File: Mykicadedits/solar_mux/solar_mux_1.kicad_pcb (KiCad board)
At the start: 2 copper layers, 122.9 x 145.3 mm, 26 parts, among them J1 Conn_01x14, U1 ASSR-1611, U10 ASSR-1611, U11 ASSR-1611, U12 ASSR-1611, U13 ASSR-1611, U14 ASSR-1611, U15 ASSR-1611, U16 ASSR-1611, U17 ASSR-1611, U2 ASSR-1611, U20 ASSR-1611, U21 ASSR-1611, U22 MCP23S17, U3 ASSR-1611, U4 ASSR-1611, U5 ASSR-1611, U6 ASSR-1611, U7 ASSR-1611

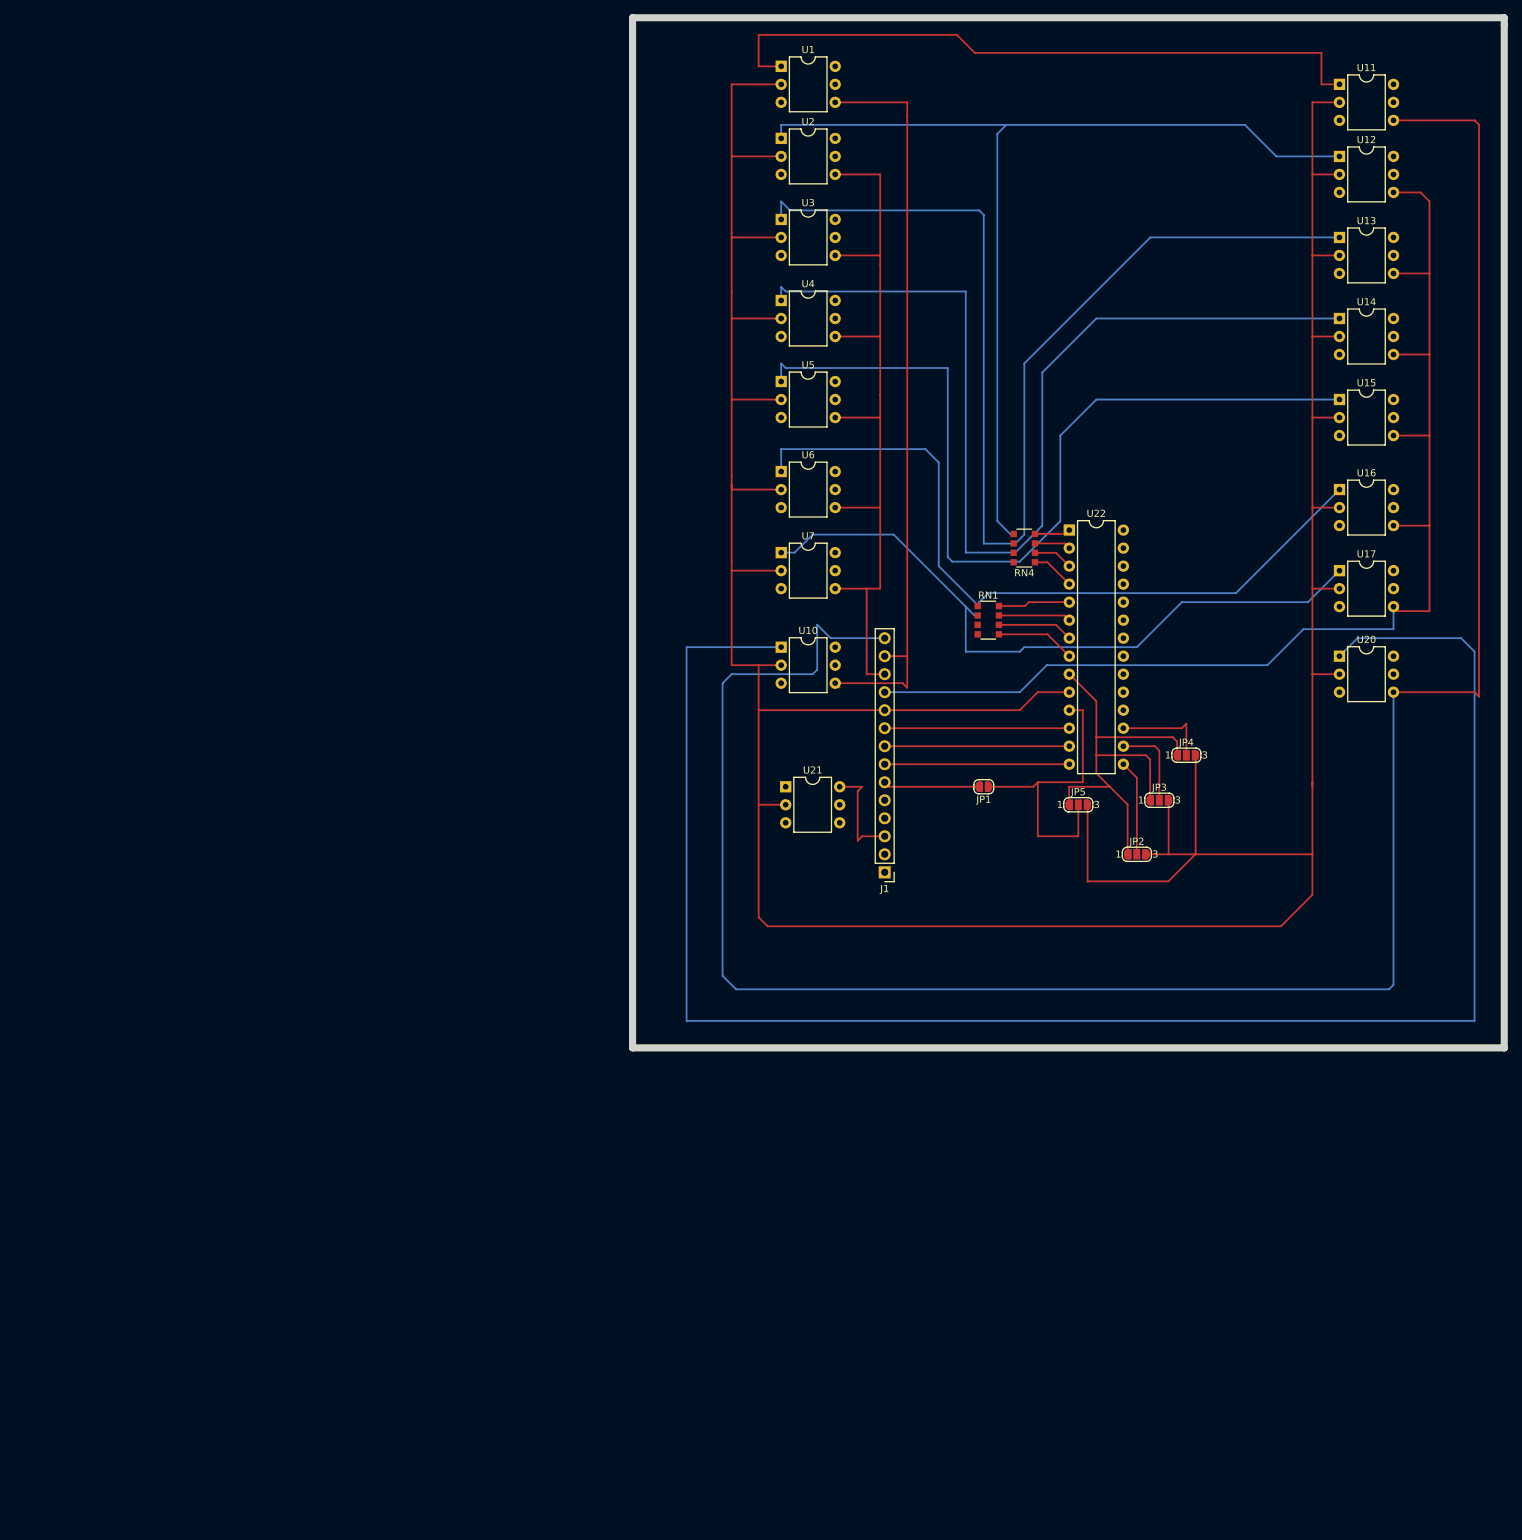
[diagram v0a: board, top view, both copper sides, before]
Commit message: Leave it!
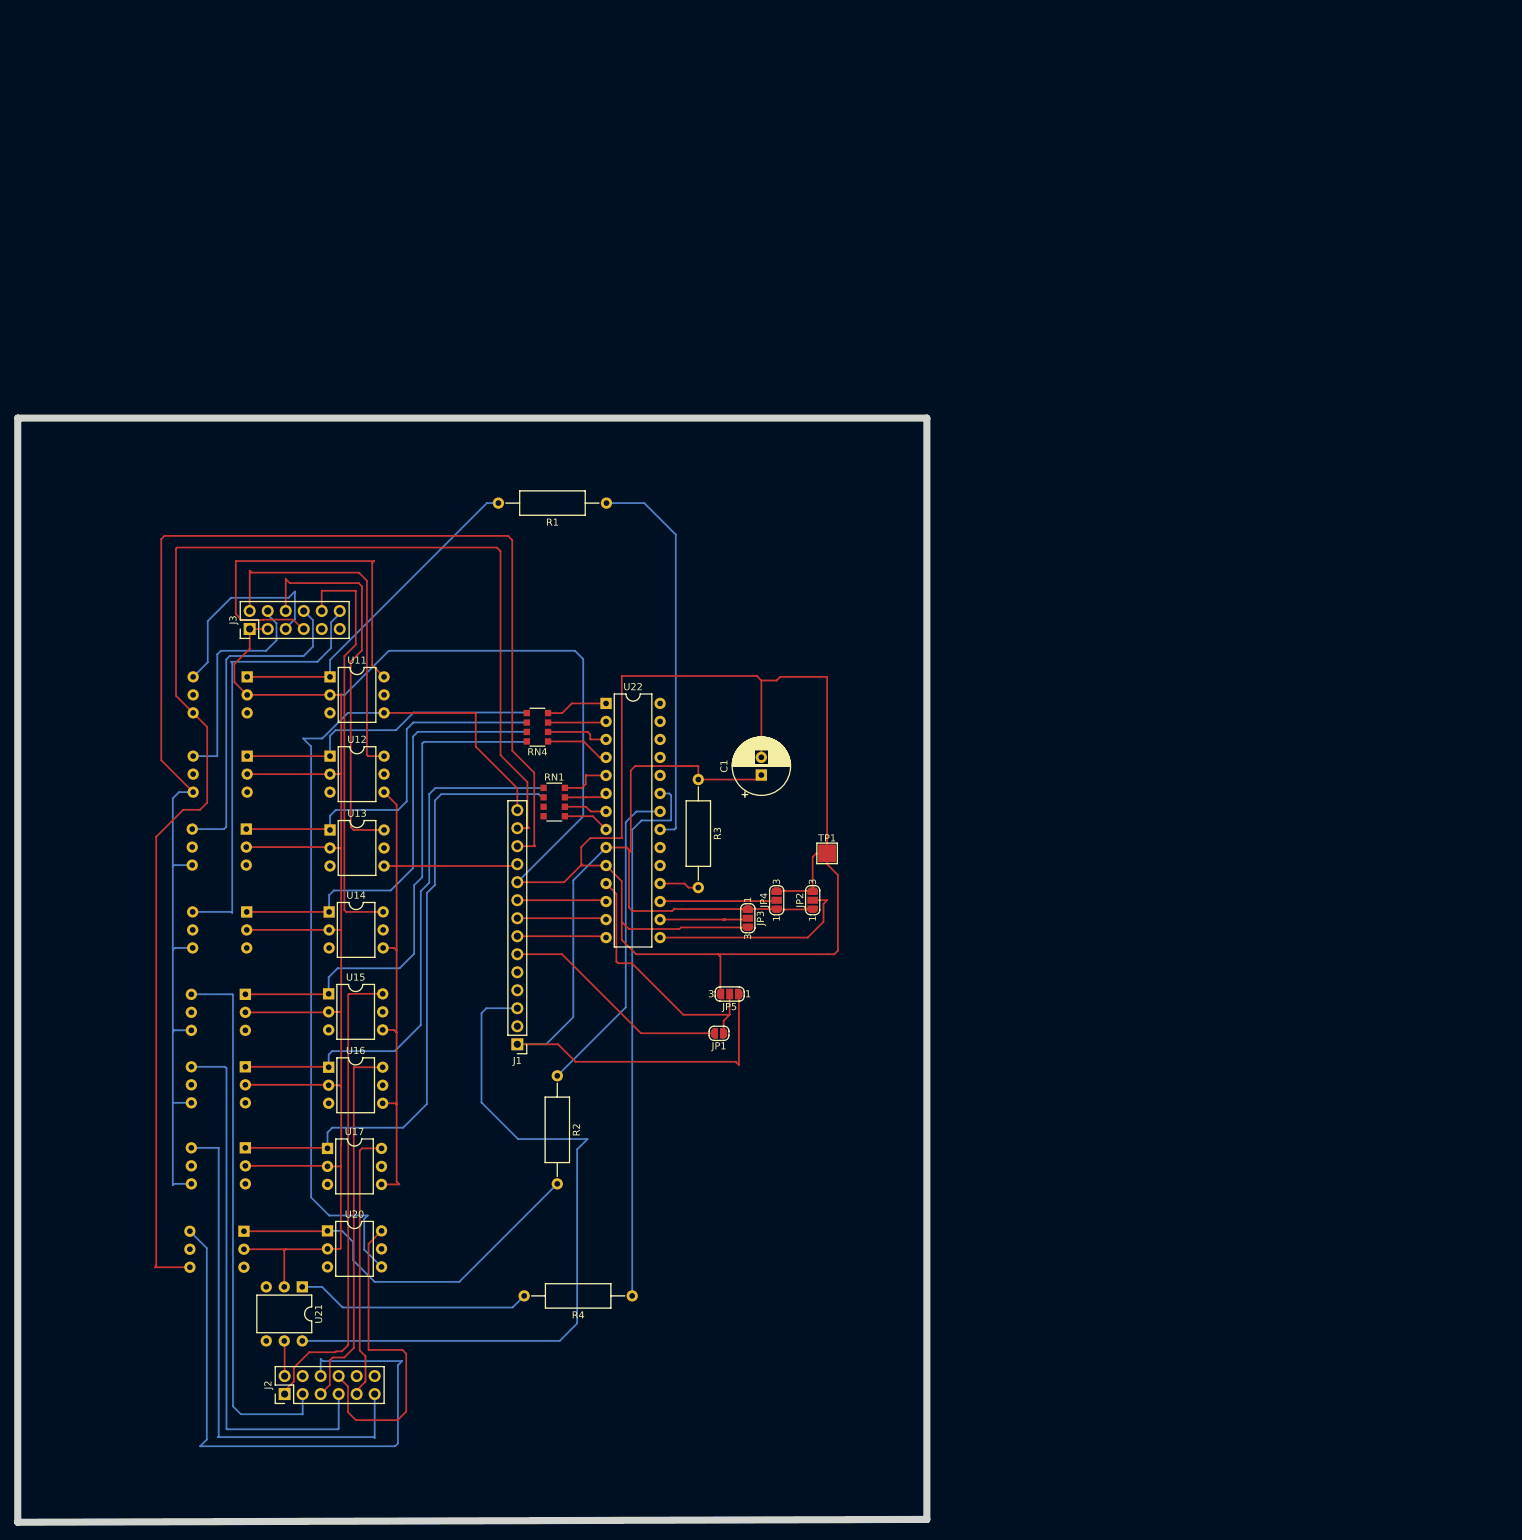
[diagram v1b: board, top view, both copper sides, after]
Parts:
- added C1: 0.1uF, Capacitor_THT:CP_Radial_D8.0mm_P2.50mm, F.Cu at (-185.0, 124.1)
- added J2: Conn_02x06_Odd_Even, Connector_PinHeader_2.54mm:PinHeader_2x06_P2.54mm_Vertical, F.Cu at (-252.3, 211.4)
- added J3: Conn_02x06_Odd_Even, Connector_PinHeader_2.54mm:PinHeader_2x06_P2.54mm_Vertical, F.Cu at (-257.2, 103.5)
- added R1: 330R, Resistor_THT:R_Axial_DIN0309_L9.0mm_D3.2mm_P15.24mm_Horizontal, F.Cu at (-206.9, 85.7)
- added R2: 330R, Resistor_THT:R_Axial_DIN0309_L9.0mm_D3.2mm_P15.24mm_Horizontal, F.Cu at (-213.8, 166.5)
- added R3: 10K, Resistor_THT:R_Axial_DIN0309_L9.0mm_D3.2mm_P15.24mm_Horizontal, F.Cu at (-193.9, 124.7)
- added R4: 680R, Resistor_THT:R_Axial_DIN0309_L9.0mm_D3.2mm_P15.24mm_Horizontal, F.Cu at (-203.3, 197.5)
- added TP1: Test_Point, TestPoint:TestPoint_Pad_2.5x2.5mm, F.Cu at (-175.8, 135.1)
- U1, U10, U2, U3, U4, U5, U6, U7: moved to B.Cu
- moved U12 165.6 mm to (-245.9, 121.4)
- moved U15 165.4 mm to (-246.1, 154.9)
- moved U14 165.3 mm to (-246.0, 143.4)
- moved U11 165.1 mm to (-245.9, 110.2)
- moved U13 165.1 mm to (-245.9, 131.8)
- moved U17 164.3 mm to (-246.2, 176.7)
- moved U16 164.2 mm to (-246.1, 165.3)
- moved U20 164.1 mm to (-246.2, 188.4)
- moved U2 115.2 mm to (-257.6, 121.4), turned to 180 degrees
- moved U5 114.8 mm to (-257.8, 155.0), turned to 180 degrees
- moved U4 114.5 mm to (-257.6, 143.4), turned to 180 degrees
- moved U1 114.4 mm to (-257.6, 110.2), turned to 180 degrees
- moved U3 114.4 mm to (-257.7, 131.7), turned to 180 degrees
- moved U6 112.9 mm to (-257.8, 165.2), turned to 180 degrees
- moved U7 112.9 mm to (-257.8, 176.7), turned to 180 degrees
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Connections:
- net /P7 renamed Net-(RN1-Pad3)
- net /P8 renamed Net-(RN1-Pad4)
- J1 pad 1: Net-(J1-Pad1) -> +5V
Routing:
- net /BOT: track 250.1 -> 54.4 mm
- net I-: track 314.3 -> 124.6 mm
- net /P2: track 160.4 -> 52.9 mm
- net /P1: track 141.6 -> 43.7 mm
- net V+: track 111.1 -> 206.1 mm
- net V-: track 107.2 -> 201.0 mm
- net V_D: track 15.1 -> 101.4 mm
- net /VB: track 0.00 -> 85.6 mm
- net +5V: track 64.2 -> 148.2 mm
- net I+: track 167.7 -> 84.2 mm
- net /P3: track 144.1 -> 62.3 mm
- net /V4: track 0.00 -> 77.1 mm
- net Net-(R4-Pad1): track 0.00 -> 77.0 mm
- net /V5: track 0.00 -> 76.7 mm
- net /V6: track 0.00 -> 73.0 mm
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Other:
- board size 122.9 x 145.3 mm -> 128.2 x 155.7 mm
